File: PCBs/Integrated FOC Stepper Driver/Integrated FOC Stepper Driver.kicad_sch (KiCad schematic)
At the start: 65 parts, among them J1 INPUT, J2 USB C Receptacle, J3 OUTPUT, J4 MOTOR, J5 Conn_01x02, SW1 BOOT, SW2 RESET, U1 PJ54M50SE, U2 PJ9500M33SA, U3 RP2040, U4 W25Q128JVS, U5 SN65HVD1050D, U6 MT6701CT, Y1 12MHz/12pF/50Ω/20ppm

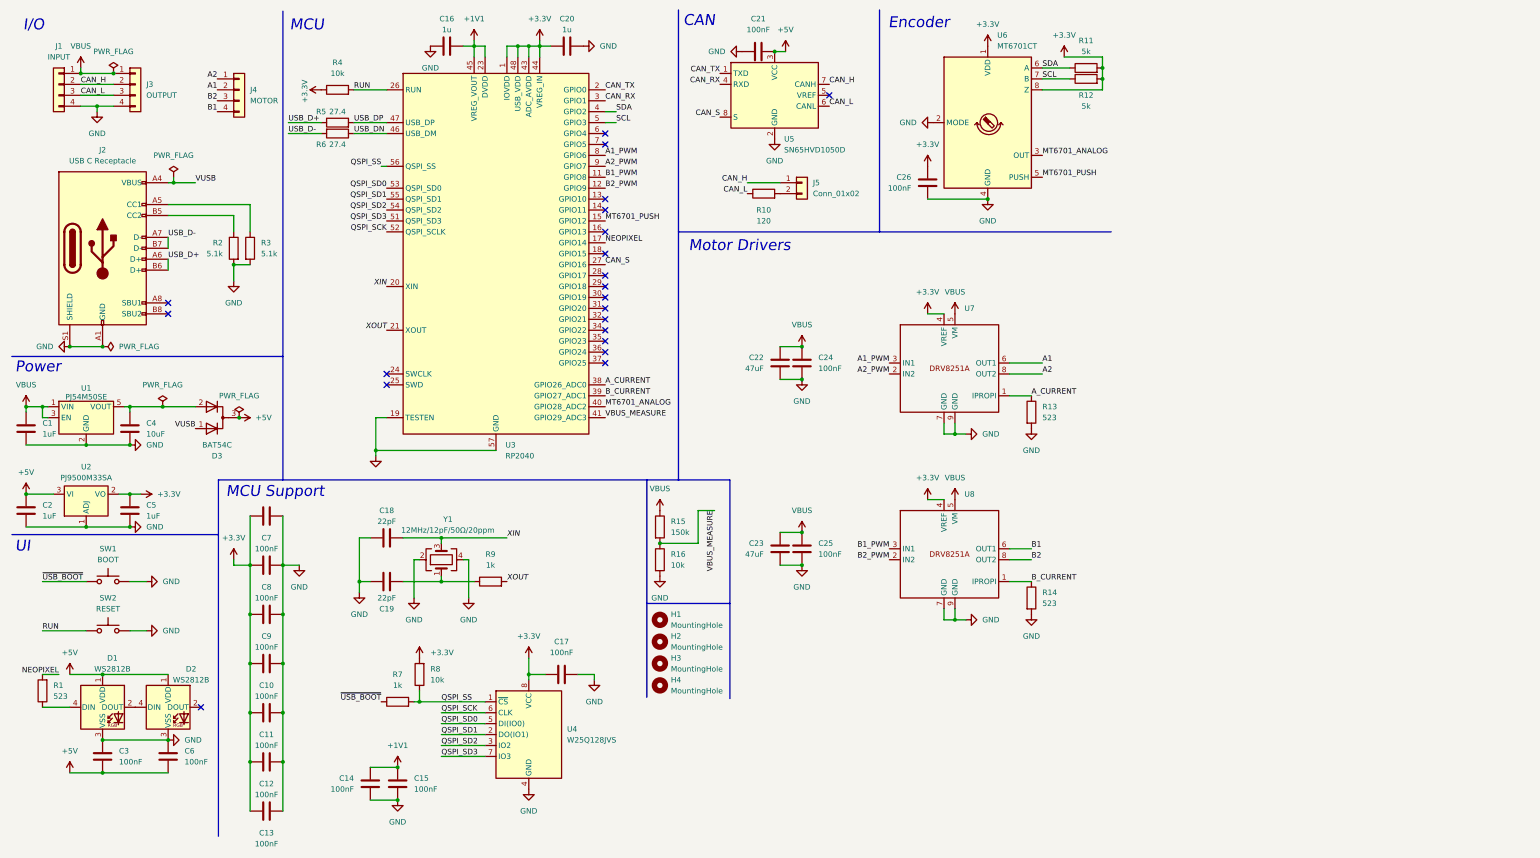
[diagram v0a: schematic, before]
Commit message: Start RP2350 design
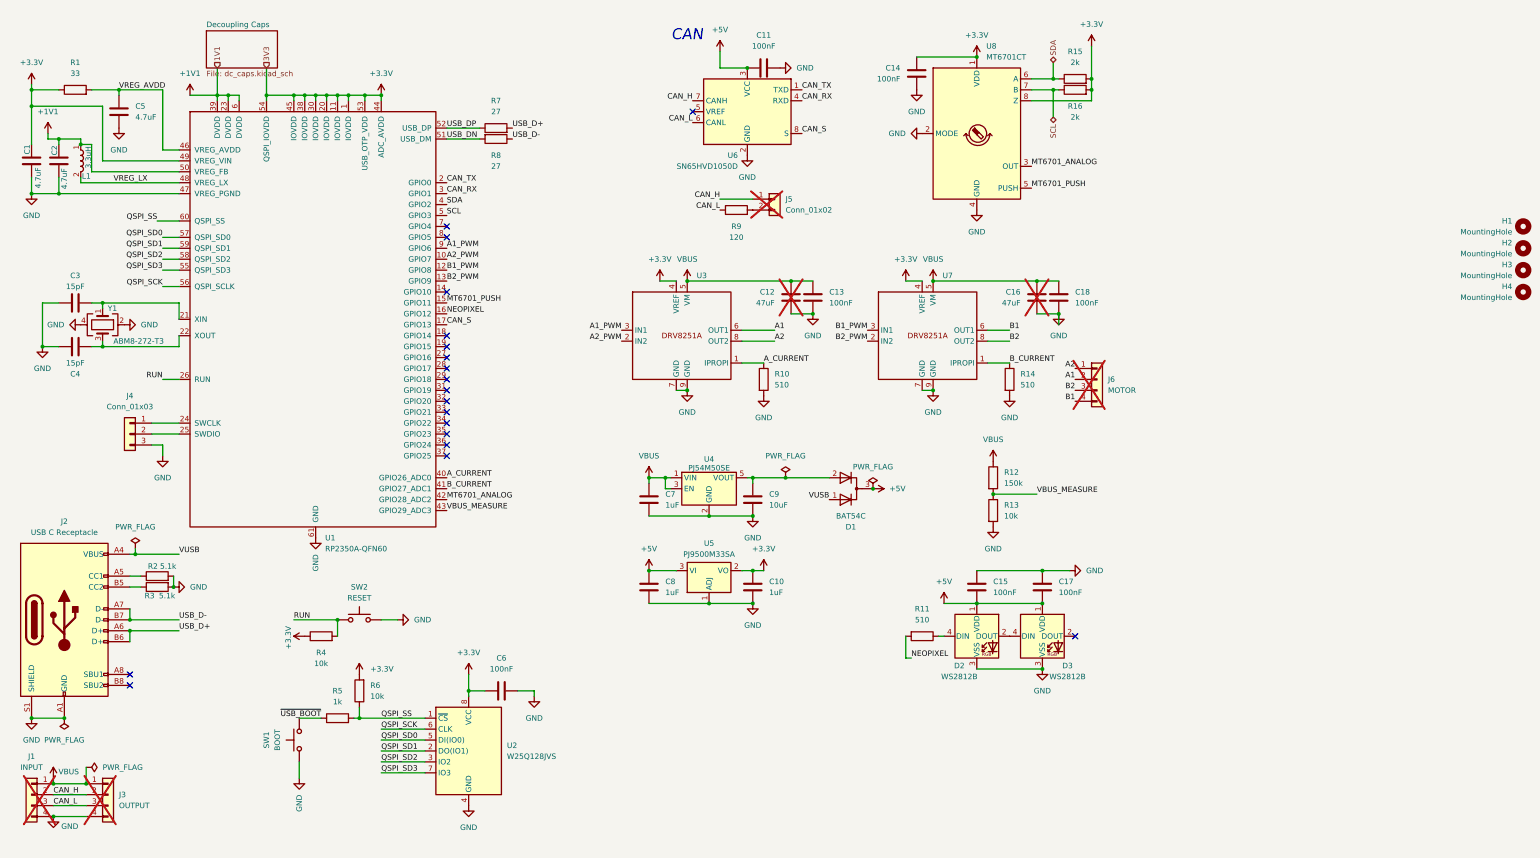
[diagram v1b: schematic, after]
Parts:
- removed C19: 22pF, Capacitor_SMD:C_0402_1005Metric, symbol Device:C
- removed C20: 1u, Capacitor_SMD:C_0402_1005Metric, symbol Device:C
- removed C21, C24, C25, C26: 100nF, Capacitor_SMD:C_0402_1005Metric, symbol Device:C
- removed C22, C23: 47uF, Capacitor_SMD:C_2220_5750Metric, symbol Device:C
- removed D1: WS2812B, LED_SMD:LED_WS2812B_PLCC4_5.0x5.0mm_P3.2mm, symbol LED:WS2812B
- removed D3: BAT54C, Package_TO_SOT_SMD:SOT-23, symbol Device:D_Dual_CommonCathode_AAK_Parallel
- removed J4: MOTOR, Connector_JST:JST_XH_S4B-XH-SM4-TB_1x04-1MP_P2.50mm_Horizontal, symbol Connector_Generic:Conn_01x04
- removed U1: PJ54M50SE, Package_TO_SOT_SMD:SOT-23-5, symbol EchoSymbols:PJ54M50SE
- removed U2: PJ9500M33SA, Package_TO_SOT_SMD:SOT-23, symbol Regulator_Linear:AMS1117
- removed U3: RP2040, Package_DFN_QFN:QFN-56-1EP_7x7mm_P0.4mm_EP3.2x3.2mm, symbol MCU_RaspberryPi:RP2040
- removed U4: W25Q128JVS, Package_SO:SOIC-8_5.23x5.23mm_P1.27mm, symbol Memory_Flash:W25Q128JVS
- removed U5: SN65HVD1050D, Package_SO:SOIC-8_3.9x4.9mm_P1.27mm, symbol Interface_CAN_LIN:SN65HVD1050D
- removed U6: MT6701CT, Package_SO:SO-8_3.9x4.9mm_P1.27mm, symbol Sensor_Magnetic:MT6701CT
- removed U8: ~, Package_SO:Texas_HSOP-8-1EP_3.9x4.9mm_P1.27mm_ThermalVias, symbol EchoSymbols:DRV8251A
- added D1: BAT54C, Package_TO_SOT_SMD:SOT-23, symbol Device:D_Dual_CommonCathode_AAK_Parallel
- added D3: WS2812B, LED_SMD:LED_WS2812B_PLCC4_5.0x5.0mm_P3.2mm, symbol LED:WS2812B
- added J4: Conn_01x03, Connector_PinHeader_2.54mm:PinHeader_1x03_P2.54mm_Vertical, symbol Connector_Generic:Conn_01x03
- added J6: MOTOR, Connector_JST:JST_XH_S4B-XH-A-1_1x04_P2.50mm_Horizontal, symbol Connector_Generic:Conn_01x04
- added L1: 3.3uH, EchoFootprints:L_0806, symbol Device:L
- added U1: RP2350A-QFN60, Package_DFN_QFN:QFN-60-1EP_7x7mm_P0.4mm_EP3.4x3.4mm_ThermalVias, symbol RP2xxx:RP2350A-QFN60
- added U2: W25Q128JVS, Package_SO:SOIC-8_5.23x5.23mm_P1.27mm, symbol Memory_Flash:W25Q128JVS
- added U3: ~, Package_SO:Texas_HSOP-8-1EP_3.9x4.9mm_P1.27mm_ThermalVias, symbol EchoSymbols:DRV8251A
- added U4: PJ54M50SE, Package_TO_SOT_SMD:SOT-23-5, symbol EchoSymbols:PJ54M50SE
- added U5: PJ9500M33SA, Package_TO_SOT_SMD:SOT-23, symbol Regulator_Linear:AMS1117
- added U6: SN65HVD1050D, Package_SO:SOIC-8_3.9x4.9mm_P1.27mm, symbol Interface_CAN_LIN:SN65HVD1050D
- added U8: MT6701CT, Package_SO:SO-8_3.9x4.9mm_P1.27mm, symbol Sensor_Magnetic:MT6701CT
- C1, C2, C5: value 1uF -> 4.7uF; footprint Capacitor_SMD:C_0603_1608Metric -> Capacitor_SMD:C_0402_1005Metric; LCSC C15849 -> (none)
- C10, C7, C8: value 100nF -> 1uF; footprint Capacitor_SMD:C_0402_1005Metric -> Capacitor_SMD:C_0603_1608Metric; LCSC C307331 -> (none)
- C11, C13, C14, C15, C17, C6: LCSC C307331 -> (none)
- C12: value 100nF -> 47uF; footprint Capacitor_SMD:C_0402_1005Metric -> Capacitor_SMD:C_2220_5750Metric; LCSC C307331 -> C5447693; now not fitted
- C16: value 1u -> 47uF; footprint Capacitor_SMD:C_0402_1005Metric -> Capacitor_SMD:C_2220_5750Metric; LCSC C29266 -> C5447693; now not fitted
- C18: value 22pF -> 100nF; LCSC C2185179 -> (none)
- C3: value 100nF -> 15pF; LCSC C307331 -> (none)
- C4: value 10uF -> 15pF; footprint Capacitor_SMD:C_0603_1608Metric -> Capacitor_SMD:C_0402_1005Metric; LCSC C96446 -> (none)
- C9: value 100nF -> 10uF; footprint Capacitor_SMD:C_0402_1005Metric -> Capacitor_SMD:C_0603_1608Metric; LCSC C307331 -> (none)
- J1, J3: now not fitted
- J5: LCSC C706874 -> (none); now not fitted
- R1: value 523 -> 33; LCSC C517803 -> C25105
- R10: value 120 -> 510; LCSC C114758 -> C25123
- R11: value 5k -> 510; LCSC C477765 -> C25123
- R12: value 5k -> 150k; LCSC C477765 -> C25755
- R13: value 523 -> 10k; LCSC C517803 -> C25744
- R14: value 523 -> 510; LCSC C517803 -> C25123
- R15: value 150k -> 2k; LCSC C93947 -> C4109
- R16: value 10k -> 2k; LCSC C60490 -> C4109
- R2, R3: LCSC C2906948 -> C25905
- R4: LCSC C60490 -> C25744
- R5: value 27.4 -> 1k; LCSC C274349 -> C11702
- R6: value 27.4 -> 10k; LCSC C274349 -> C25744
- R7: value 1k -> 27; LCSC C106235 -> C25100
- R8: value 10k -> 27; LCSC C60490 -> C25100
- R9: value 1k -> 120; LCSC C106235 -> C25079
- Y1: value 12MHz/12pF/50Ω/20ppm -> ABM8-272-T3; LCSC C258938 -> C20625731
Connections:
- net XOUT is gone; now on an unnamed net: R9.2
- net +1V1: now also C2.2, L1.1, U1.23 (DVDD), U1.39 (DVDD), U1.50 (VREG_FB), U1.6 (DVDD); no longer C14.2, C15.2, C16.2
- net +3.3V: now also C1.2, C10.1, C14.1, C6.1, R1.1, R15.2, R16.2, R6.2, U1.1 (IOVDD), U1.11 (IOVDD), U1.20 (IOVDD), U1.30 (IOVDD), U1.38 (IOVDD), U1.44 (ADC_AVDD), U1.45 (IOVDD), U1.49 (VREG_VIN), U1.53 (USB_OTP_VDD), U1.54 (QSPI_IOVDD), U2.8 (VCC), U3.4 (VREF), U5.2 (VO), U8.1 (VDD), U8.8 (Z); no longer C10.2, C11.2, C12.2, C13.2, C17.1, C5.1, C7.2, C8.2, C9.2, R11.2, R12.2, R8.2
- net +5V: now also C11.1, C15.1, C17.1, C8.1, D1.3 (K), D3.1 (VDD), U5.3 (VI), U6.3 (VCC); no longer C2.1, C3.1, C6.1
- net A1: now also J6.2 (Pin_2), U3.6 (OUT1); no longer U7.6 (OUT1)
- net A1_PWM: now also U1.9 (GPIO6), U3.3 (IN1); no longer U7.3 (IN1)
- net A2: now also J6.1 (Pin_1), U3.8 (OUT2); no longer U7.8 (OUT2)
- net A2_PWM: now also U1.10 (GPIO7), U3.2 (IN2); no longer U7.2 (IN2)
- net A_CURRENT: now also R10.1, U1.40 (GPIO26_ADC0), U3.1 (IPROPI); no longer R13.1, U7.1 (IPROPI)
- net B1: now also U7.6 (OUT1), J6.4 (Pin_4)
- net B1_PWM: now also U7.3 (IN1), U1.12 (GPIO8)
- net B2: now also U7.8 (OUT2), J6.3 (Pin_3)
- net B2_PWM: now also U7.2 (IN2), U1.13 (GPIO9)
- net B_CURRENT: now also U7.1 (IPROPI), U1.41 (GPIO27_ADC1)
- net CAN_H: now also U6.7 (CANH)
- net CAN_L: now also R9.1, U6.6 (CANL); no longer R10.1
- net CAN_RX: now also U1.3 (GPIO1), U6.4 (RXD)
- net CAN_S: now also U1.17 (GPIO13), U6.8 (S)
- net CAN_TX: now also U1.2 (GPIO0), U6.1 (TXD)
- net GND: now also C1.1, C10.2, C11.2, C12.2, C13.2, C14.2, C15.2, C16.2, C18.2, C2.1, C3.1, C5.1, C7.2, C8.2, C9.2, R10.2, D3.3 (VSS), J4.3 (Pin_3), U1.47 (VREG_PGND), U1.61 (GND), U2.4 (GND), U3.7 (GND), U3.9 (GND), U4.2 (GND), U5.1 (ADJ), U6.2 (GND), U8.2 (MODE), U8.4 (GND); no longer C1.2, C10.1, C11.1, C12.1, C13.1, C14.1, C15.1, C16.1, C18.1, C2.2, C3.2, C5.2, C7.1, C8.1, C9.1, R16.2
- net MT6701_ANALOG: now also U1.42 (GPIO28_ADC2), U8.3 (OUT)
- net MT6701_PUSH: now also U1.15 (GPIO11), U8.5 (PUSH)
- net NEOPIXEL: now also R11.2, U1.16 (GPIO12); no longer R1.2
- net QSPI_SCK: now also U1.56 (QSPI_SCLK), U2.6 (CLK)
- net QSPI_SD0: now also U1.57 (QSPI_SD0), U2.5 (DI(IO0))
- net QSPI_SD1: now also U1.59 (QSPI_SD1), U2.2 (DO(IO1))
- net QSPI_SD2: now also U1.58 (QSPI_SD2), U2.3 (IO2)
- net QSPI_SD3: now also U1.55 (QSPI_SD3), U2.7 (IO3)
- net QSPI_SS: now also R5.2, R6.1, U1.60 (QSPI_SS), U2.1 (~{CS}); no longer R7.2, R8.1
- net RUN: now also U1.26 (RUN)
- net SCL: now also R16.1, U1.5 (GPIO3), U8.7 (B); no longer R12.1
- net SDA: now also R15.1, U1.4 (GPIO2), U8.6 (A); no longer R11.1
- net USB_D+: now also R7.2; no longer R5.1
- net USB_D-: now also R8.1; no longer R6.2
- net USB_DN: now also R8.2, U1.51 (USB_DM); no longer R6.1
- net USB_DP: now also R7.1, U1.52 (USB_DP); no longer R5.2
- net VBUS: now also C12.1, C13.1, C16.1, C18.1, C7.1, R12.1, U3.5 (VM), U4.1 (VIN), U4.3 (EN); no longer C1.1, R15.1
- net VBUS_MEASURE: now also R12.2, R13.1, U1.43 (GPIO29_ADC3); no longer R15.2, R16.1
- net VUSB: now also D1.1 (A)
- net ~{USB_BOOT}: now also R5.1; no longer R7.1
- net at J2.A5 (CC1): now also R2.1; no longer R3.1
- net at J2.B5 (CC2): now also R3.1; no longer R2.1
- net at C4.1: now also Y1.3, U1.22 (XOUT)
- net at D2.4 (DIN): now also R11.1
- net at Y1.1: now also C3.2, U1.21 (XIN); no longer R9.1
- net at J5.2 (Pin_2): no longer R10.2
- net at D2.2 (DOUT): now also D3.4 (DIN)
- removed net XIN: C18.2, Y1.3
- new net: J4.1 (Pin_1), U1.24 (SWCLK)
- new net: J4.2 (Pin_2), U1.25 (SWDIO)
- new net: C9.1, D1.2 (A), U4.5 (VOUT)
- new net VREG_AVDD: C5.2, R1.2, U1.46 (VREG_AVDD)
- new net VREG_LX: L1.2, U1.48 (VREG_LX)
- no-connect marks 21 -> 19
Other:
- added sheet Decoupling Caps (dc_caps.kicad_sch)
- note removed: "Encoder"
- note removed: "I/O"
- note removed: "MCU"
- note removed: "MCU Support"
- note removed: "Motor Drivers"
- note removed: "Power"
- note removed: "UI"
